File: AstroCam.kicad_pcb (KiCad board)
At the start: 2 copper layers, 115 x 40 mm, 114 parts, among them P1 CONN_01X02, P2 CONN_01X08, P3 CONN_02X12, Q1 Q_NMOS_DGS, U1 LMZ10500, U10 CXD3400N, U11 ICX825AQA, U12 ADDI7013, U3 TPS2420, U5 LM3674, U6 TPS56x200, U7 TPS56x200, U8 TPS56x200, U9 LMR62014

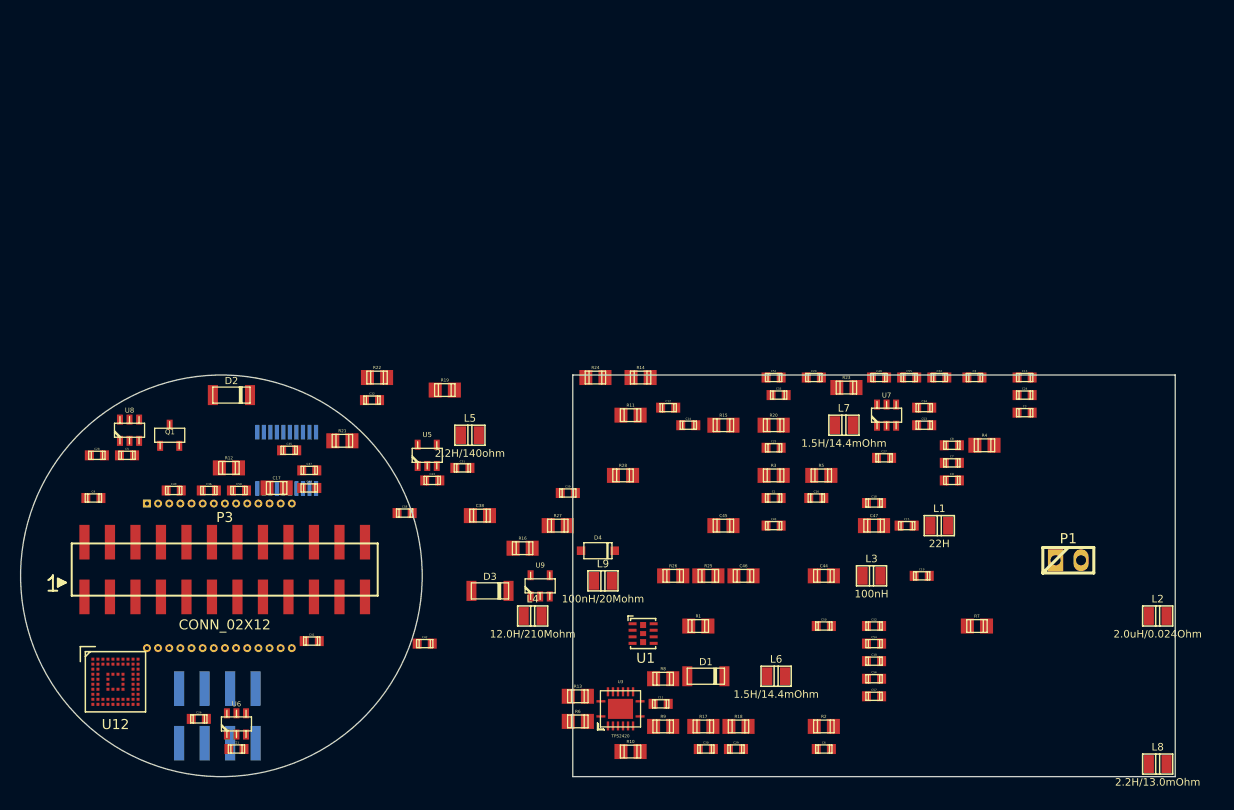
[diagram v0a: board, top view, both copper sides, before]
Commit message: More work on schematic
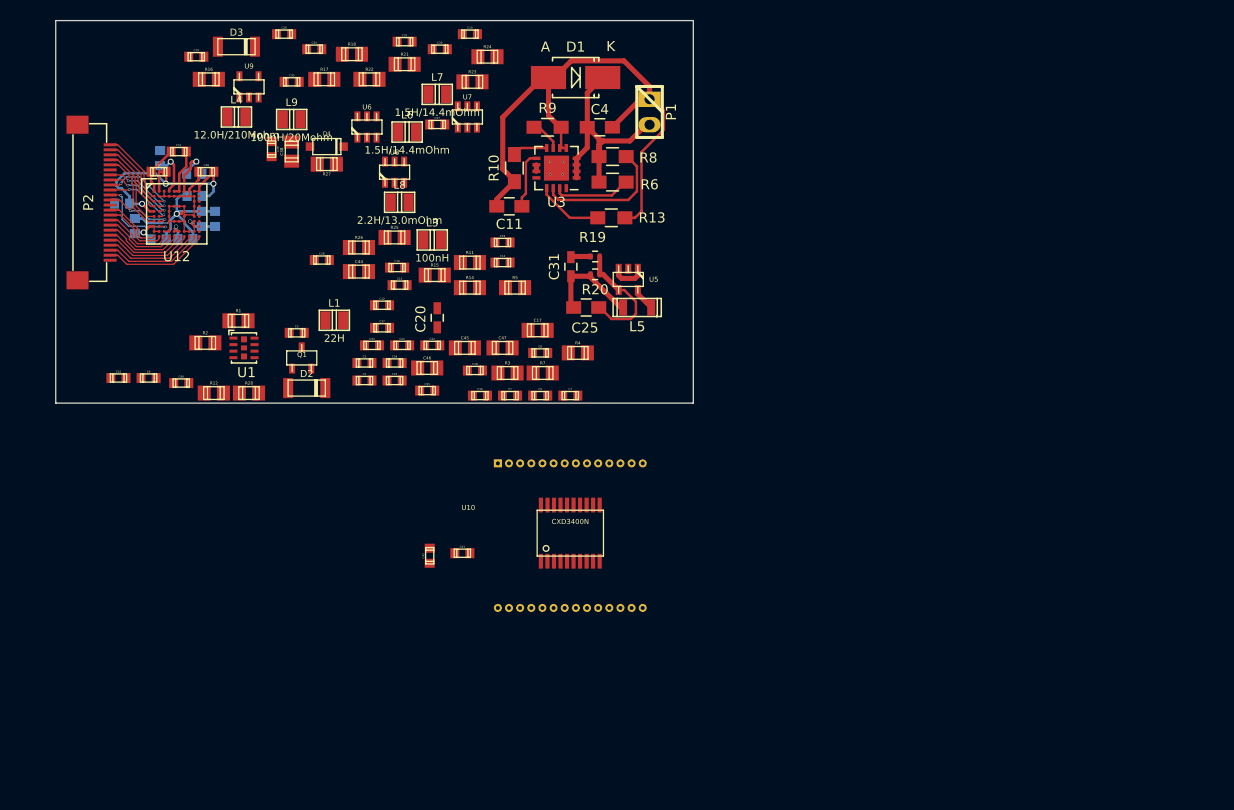
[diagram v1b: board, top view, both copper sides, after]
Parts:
- removed L2: 2.0uH/0.024Ohm, w_smd_inductors:inductor_smd_0805
- removed P3: CONN_02X12, w_smd_strip:bb02-hp24
- C11, C25, C4: footprint w_smd_cap:c_0603 -> Capacitors_SMD:C_0805_HandSoldering
- C20, C31: footprint w_smd_cap:c_0603 -> Capacitors_SMD:C_0603_HandSoldering
- C39: value 0.1u -> 0.1uF
- C40: value 2200pF -> 2.2uF
- C49, C52, C53, C54, C55, C56, C57, C58, C59: moved to B.Cu
- D1: footprint w_smd_diode:sod80c -> Diodes_SMD:Diode-SMB_Handsoldering
- L5: footprint w_smd_inductors:inductor_smd_0805 -> camera:Inductor_SMD_2016
- P2: value CONN_01X08 -> CONN_01X24; footprint w_smd_strip:bb02-hp08 -> camera:FFC-24-0.5mm; moved to F.Cu
- R10, R13, R6, R8, R9: footprint w_smd_resistors:r_0805 -> Resistors_SMD:R_0805_HandSoldering
- R19, R20: footprint w_smd_resistors:r_0805 -> Resistors_SMD:R_0402
- U10: moved to F.Cu
- U3: footprint w_smd_qfn:pvqfn-n16 -> Housings_DFN_QFN:QFN-16-1EP_4x4mm_Pitch0.65mm
- moved L8 94.0 mm to (117.8, 112.8)
- moved C56 88.6 mm to (90.1, 112.9)
- moved C29 87.4 mm to (97.5, 98.3)
- moved C53 81.1 mm to (91.4, 115.2), turned to 270 degrees
- moved C57 81.0 mm to (99.4, 114.5), turned to 270 degrees
- moved C50 80.2 mm to (93.8, 109.8)
- moved C52 80.1 mm to (97.3, 112.2)
- moved C15 79.9 mm to (89.8, 130.3)
- moved C54 79.2 mm to (98.0, 114.5), turned to 270 degrees
- moved C30 78.2 mm to (107.0, 100.8)
- moved R18 77.2 mm to (113.0, 98.0)
- moved C6 76.7 mm to (92.8, 130.3)
- moved R17 74.7 mm to (110.2, 100.5)
- moved C10 74.3 mm to (124.8, 96.0)
- moved C55 73.4 mm to (96.4, 116.5), turned to 180 degrees
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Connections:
- C55 pad 1: /camera/GND -> /h-driver/1V8
- C55 pad 2: /h-driver/1V8 -> /camera/GND
- P2 pad 1: Net-(P2-Pad1) -> /h-driver/CLI
- P2 pad 2: Net-(P2-Pad2) -> /h-driver/GP01
- P2 pad 3: Net-(P2-Pad3) -> /h-driver/GP02
- P2 pad 4: Net-(P2-Pad4) -> /h-driver/GP03
- P2 pad 5: Net-(P2-Pad5) -> /h-driver/GP04
- P2 pad 6: Net-(P2-Pad6) -> /camera/GND
- P2 pad 7: Net-(P2-Pad7) -> /h-driver/SCK
- P2 pad 8: /camera/GND -> /h-driver/SDATA
- U10 pad 10: Net-(P2-Pad7) -> /camera/XV4
- U10 pad 12: /camera/VT1 -> /camera/VT4
- U10 pad 13: /camera/VT2 -> /camera/VT1
- U10 pad 17: /camera/VT4 -> /camera/VT2
- U10 pad 2: Net-(P2-Pad1) -> /camera/XSHT
- U10 pad 3: Net-(P2-Pad2) -> /camera/XV2
- U10 pad 5: Net-(P2-Pad3) -> /camera/XSGV2
- U10 pad 6: Net-(P2-Pad4) -> /camera/XV3
- U10 pad 8: Net-(P2-Pad5) -> /camera/XSGV3
- U10 pad 9: Net-(P2-Pad6) -> /camera/XV1
- U12 pad B1: Net-(P3-Pad23) -> /h-driver/CLI
- U12 pad C1: Net-(P3-Pad21) -> /h-driver/GP01
- U12 pad C2: Net-(P3-Pad3) -> /h-driver/SL
- U12 pad D1: Net-(P3-Pad19) -> /h-driver/GP02
- U12 pad D2: Net-(P3-Pad7) -> /h-driver/SCK
- U12 pad D6: (no net) -> /camera/GND
- U12 pad E2: Net-(P3-Pad5) -> /h-driver/SDATA
- U12 pad F1: Net-(P3-Pad17) -> /h-driver/GP03
- U12 pad F2: Net-(P3-Pad13) -> /h-driver/SYNC
- U12 pad G1: Net-(P3-Pad15) -> /h-driver/GP04
- U12 pad G2: Net-(P3-Pad9) -> /h-driver/HD
- U12 pad H2: Net-(P3-Pad11) -> /h-driver/VD
- U12 pad K1: Net-(P3-Pad24) -> /h-driver/A0+
- U12 pad K10: Net-(P3-Pad2) -> /h-driver/B1-
- U12 pad K2: Net-(P3-Pad22) -> /h-driver/A0-
- U12 pad K3: Net-(P3-Pad20) -> /h-driver/A1+
- U12 pad K4: Net-(P3-Pad18) -> /h-driver/A1-
- U12 pad K5: Net-(P3-Pad14) -> /h-driver/TCLK+
- U12 pad K6: Net-(P3-Pad12) -> /h-driver/TCLK-
- U12 pad K7: Net-(P3-Pad8) -> /h-driver/B0+
- U12 pad K8: Net-(P3-Pad6) -> /h-driver/B0-
- U12 pad K9: Net-(P3-Pad4) -> /h-driver/B1+
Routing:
- net /camera/GND: track 0.00 -> 101.7 mm, vias 0 -> 1
- net /h-driver/3V3: track 0.00 -> 31.1 mm, vias 0 -> 4
- net /power-supply/V_BATT: track 0.00 -> 24.0 mm
- net Net-(R8-Pad2): track 0.00 -> 13.5 mm
- net Net-(C25-Pad2): track 0.00 -> 12.1 mm
- net /h-driver/1V8: track 0.00 -> 12.1 mm, vias 0 -> 2
- net /h-driver/B1-: track 0.00 -> 10.5 mm
- net /power-supply/2V5: track 0.00 -> 10.1 mm
- net /h-driver/B1+: track 0.00 -> 9.99 mm
- net /h-driver/B0-: track 0.00 -> 9.44 mm
- net /h-driver/B0+: track 0.00 -> 8.92 mm
- net /h-driver/VD: track 0.00 -> 8.90 mm, vias 0 -> 2
- net /h-driver/TCLK-: track 0.00 -> 8.38 mm
- net /h-driver/GP03: track 0.00 -> 8.33 mm
- net /h-driver/GP04: track 0.00 -> 8.33 mm
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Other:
- board size 115 x 40 mm -> 63.5 x 38.1 mm
- rule trace_min: 0.2 -> 0.1
- rule via_min_drill: 0.3 -> 0.1
- rule via_min_size: 0.4 -> 0.1
